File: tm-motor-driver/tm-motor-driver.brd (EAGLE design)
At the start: 44 x 24 mm, 18 parts

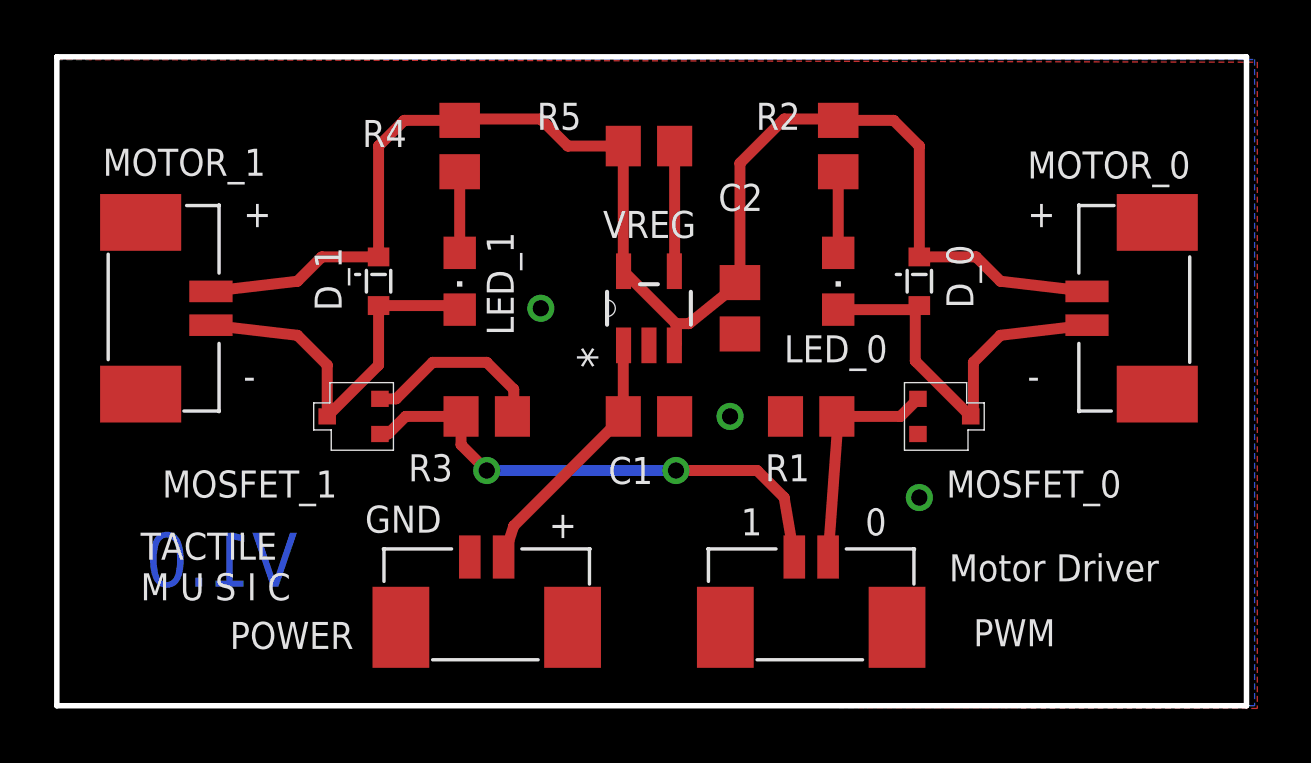
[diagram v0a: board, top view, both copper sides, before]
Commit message: Generate gerber files
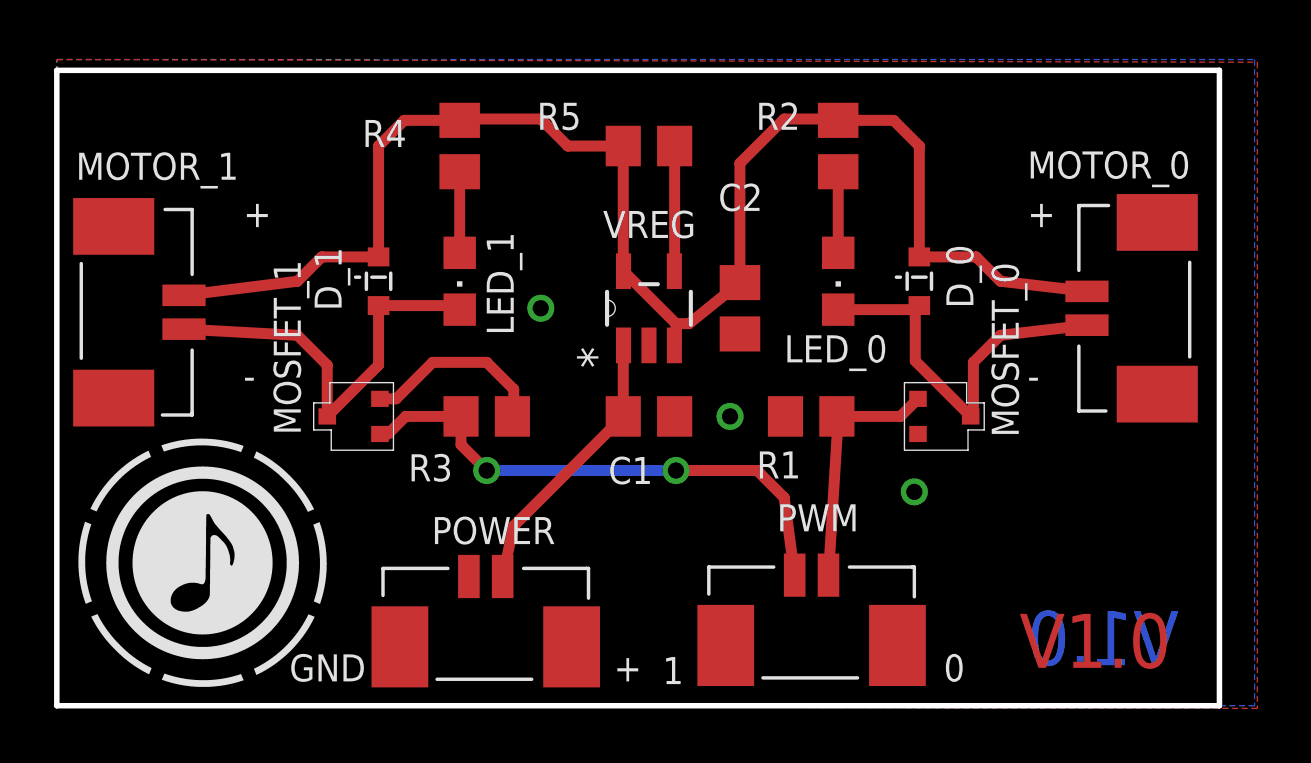
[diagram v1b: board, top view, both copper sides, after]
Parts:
- moved MOTOR_1 1.01 mm to (2.90, 14.6)
- moved POWER 0.72 mm to (15.9, 2.98)
- moved PWM 0.67 mm to (27.9, 3.03)
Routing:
- net +3V3: track 55.0 -> 56.0 mm
- net N$1: track 14.6 -> 15.6 mm
- net BATT_V+: track 9.58 -> 10.3 mm
- net PWM0: track 8.50 -> 9.17 mm
- net PWM1: track 19.3 -> 20.0 mm
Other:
- board size 44 x 24 mm -> 43 x 23.5 mm
- board text added: "C:/EAGLE-7.6.0/lbr/tactile-music-hw-lib/ICON.bmp"
- board text removed: "Motor Driver"
- board text removed: "TACTILE M U S I C"
